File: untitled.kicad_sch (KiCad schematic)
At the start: 14 parts, among them SW1 SW_Push, U1 ATmega328P-A, Y1 16MHz

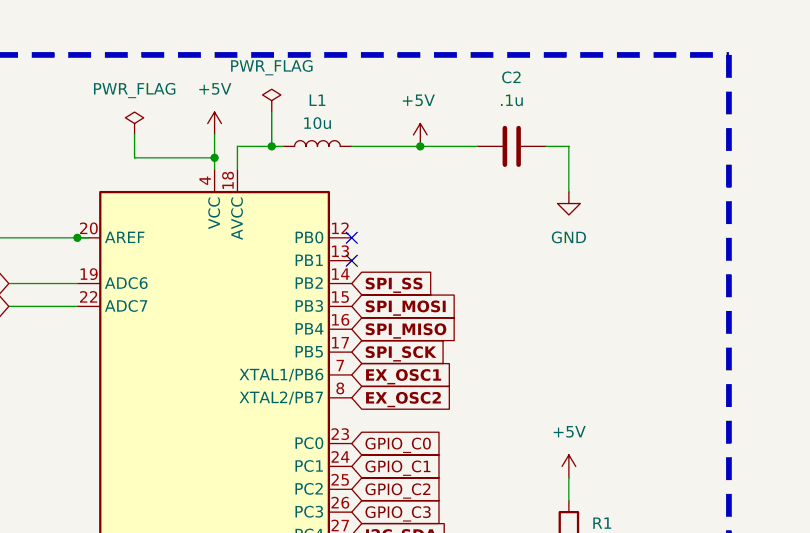
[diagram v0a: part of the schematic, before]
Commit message: final intro pcb
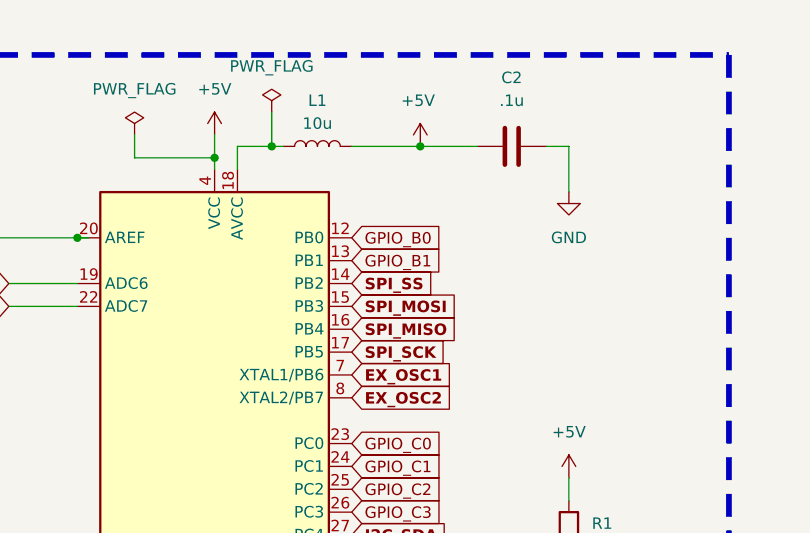
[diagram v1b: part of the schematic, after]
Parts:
- C3, C4: footprint Capacitor_SMD:C_0402_1005Metric_Pad0.74x0.62mm_HandSolder -> Capacitor_SMD:C_0603_1608Metric_Pad1.08x0.95mm_HandSolder
- L1: footprint (none) -> Inductor_SMD:L_0603_1608Metric_Pad1.05x0.95mm_HandSolder
- R1, R2, R3, R4: footprint (none) -> Resistor_SMD:R_0402_1005Metric_Pad0.72x0.64mm_HandSolder
- SW1: footprint (none) -> Button_Switch_SMD:SW_Push_SPST_NO_Alps_SKRK
- Y1: footprint (none) -> Crystal:Crystal_SMD_2012-2Pin_2.0x1.2mm_HandSoldering
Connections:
- net GPIO_B0: now reaches U1.12 (PB0)
- net GPIO_B1: now reaches U1.13 (PB1)
- no-connect marks 2 -> 0
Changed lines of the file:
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@@
 		(color 0 0 0 0)
 	)
-	(no_connect
-		(at 86.36 49.53)
-	)
-	(no_connect
-		(at 86.36 46.99)
-	)
 	(wire
 		(pts
@@
 		)
 	)
+	(global_label "GPIO_B1"
+		(shape input)
+		(at 86.36 49.53 0)
+		(fields_autoplaced yes)
+		(effects
+			(font
+				(size 1.27 1.27)
+			)
+			(justify left)
+		)
+		(property "Intersheetrefs" "${INTERSHEET_REFS}"
+			(at 97.2676 49.53 0)
+			(effects
+				(font
+					(size 1.27 1.27)
+				)
+				(justify left)
+				(hide yes)
+			)
+		)
+	)
 	(global_label "SPI_SS"
 		(shape input)
@@
 		)
 	)
+	(global_label "GPIO_B0"
+		(shape input)
+		(at 86.36 46.99 0)
+		(fields_autoplaced yes)
+		(effects
+			(font
+				(size 1.27 1.27)
+			)
+			(justify left)
+		)
+		(property "Intersheetrefs" "${INTERSHEET_REFS}"
+			(at 97.2676 46.99 0)
+			(effects
+				(font
+					(size 1.27 1.27)
+				)
+				(justify left)
+				(hide yes)
+			)
+		)
+	)
 	(global_label "GPIO_C0"
 		(shape input)
@@
 			)
 		)
-		(property "Footprint" ""
+		(property "Footprint" "Inductor_SMD:L_0603_1608Metric_Pad1.05x0.95mm_HandSolder"
 			(at 82.55 36.83 0)
 			(effects
@@
 			)
 		)
-		(property "Footprint" "Capacitor_SMD:C_0402_1005Metric_Pad0.74x0.62mm_HandSolder"
+		(property "Footprint" "Capacitor_SMD:C_0603_1608Metric_Pad1.08x0.95mm_HandSolder"
 			(at 155.9052 46.99 0)
 			(effects
@@
 			)
 		)
-		(property "Footprint" ""
+		(property "Footprint" "Resistor_SMD:R_0402_1005Metric_Pad0.72x0.64mm_HandSolder"
 			(at 159.512 133.35 90)
 			(effects
@@
 			)
 		)
-		(property "Footprint" ""
+		(property "Footprint" "Button_Switch_SMD:SW_Push_SPST_NO_Alps_SKRK"
 			(at 214.63 30.48 0)
 			(effects
@@
 			)
 		)
-		(property "Footprint" ""
+		(property "Footprint" "Resistor_SMD:R_0402_1005Metric_Pad0.72x0.64mm_HandSolder"
 			(at 169.672 133.35 90)
 			(effects
@@
 			)
 		)
-		(property "Footprint" ""
+		(property "Footprint" "Crystal:Crystal_SMD_2012-2Pin_2.0x1.2mm_HandSoldering"
 			(at 181.61 85.09 0)
 			(effects
@@
 			)
 		)
-		(property "Footprint" ""
+		(property "Footprint" "Resistor_SMD:R_0402_1005Metric_Pad0.72x0.64mm_HandSolder"
 			(at 108.712 80.01 90)
 			(effects
@@
 			)
 		)
-		(property "Footprint" "Capacitor_SMD:C_0402_1005Metric_Pad0.74x0.62mm_HandSolder"
+		(property "Footprint" "Capacitor_SMD:C_0603_1608Metric_Pad1.08x0.95mm_HandSolder"
 			(at 172.4152 46.99 0)
 			(effects
@@
 			)
 		)
-		(property "Footprint" ""
+		(property "Footprint" "Resistor_SMD:R_0402_1005Metric_Pad0.72x0.64mm_HandSolder"
 			(at 164.592 85.09 90)
 			(effects
